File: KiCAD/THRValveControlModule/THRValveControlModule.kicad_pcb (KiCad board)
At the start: 2 copper layers, 99 x 75 mm, 54 parts, among them J1 B4B-XH-A(LF)(SN), J2 B3B-XH-A(LF)(SN), J3 B3B-XH-A(LF)(SN), J4 XT30PW-M, J5 DF51A-4P-2DSA, J6 SSD1306, J7 DF51A-8DP-2DS, Q1 IRLML6344TRPBFTR, U1 XIAO-RA4M1-SMD, U10 MB85RQ8MX, U2 ICM-42688, U3 ADXL375, U4 ATA6561, U5 MAX485E, U6 SC8721, U7 BP5293-50, U8 TC7S14F, U9 TC7S14F

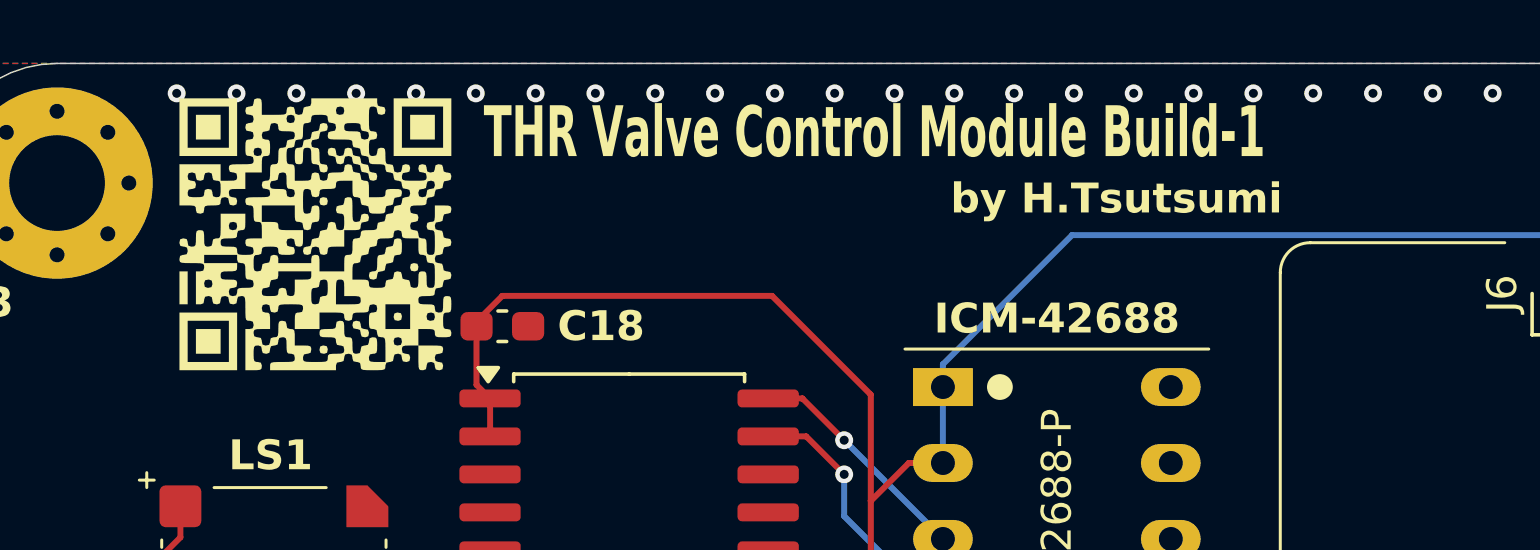
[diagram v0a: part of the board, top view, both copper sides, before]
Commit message: 基板発注完了
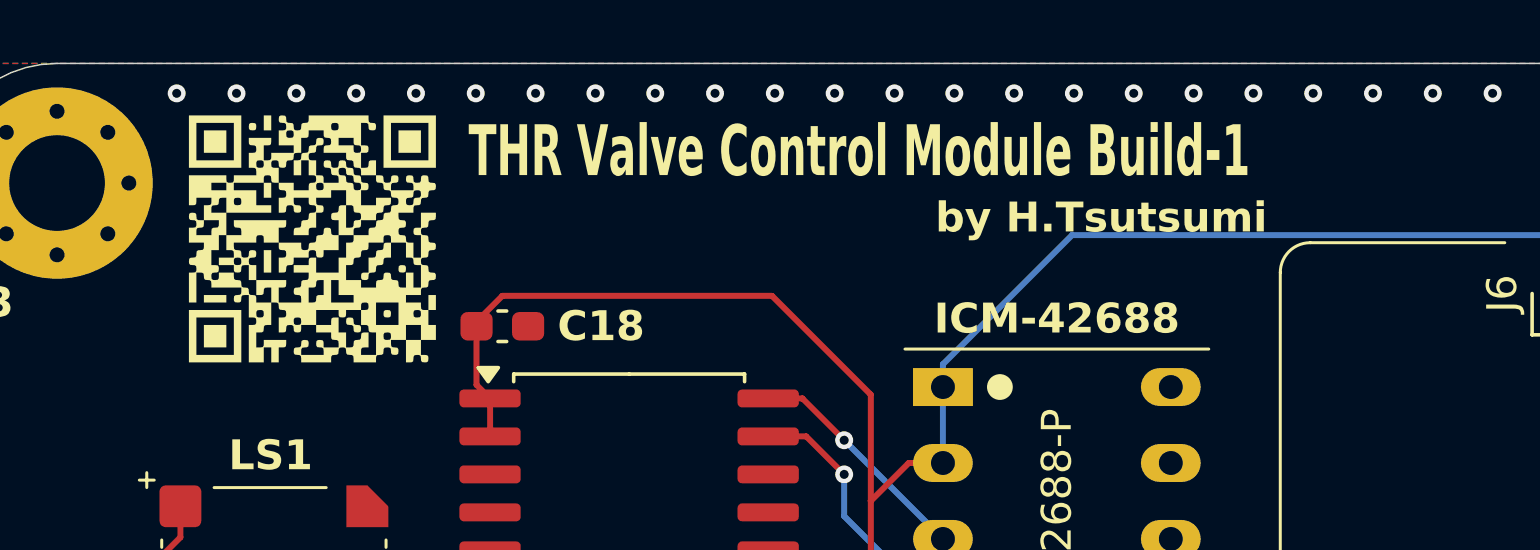
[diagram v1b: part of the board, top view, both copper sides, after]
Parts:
- moved G*** 0.18 mm to (113.5, 78.9)
